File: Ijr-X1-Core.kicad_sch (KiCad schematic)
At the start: 67 parts, among them J1 USB-C_PWR_IN, J2 USB-C_CPU_PROG, J3 USB-C_UART_BRIDGE, Q1 BSC010NE2LS, Q2 BSC010NE2LS, Q3 BSC010NE2LS, Q4 BSC010NE2LS, Q5 BSC010NE2LS, Q6 BSC010NE2LS, Q7 BSC010NE2LS, Q8 BSC010NE2LS, U1 RP2040, U2 W25Q16JVSSIQ, U3 ISL8117FRZ, U4 ISL8117FRZ, U5 ISL8117FRZ, U6 ISL8117FRZ

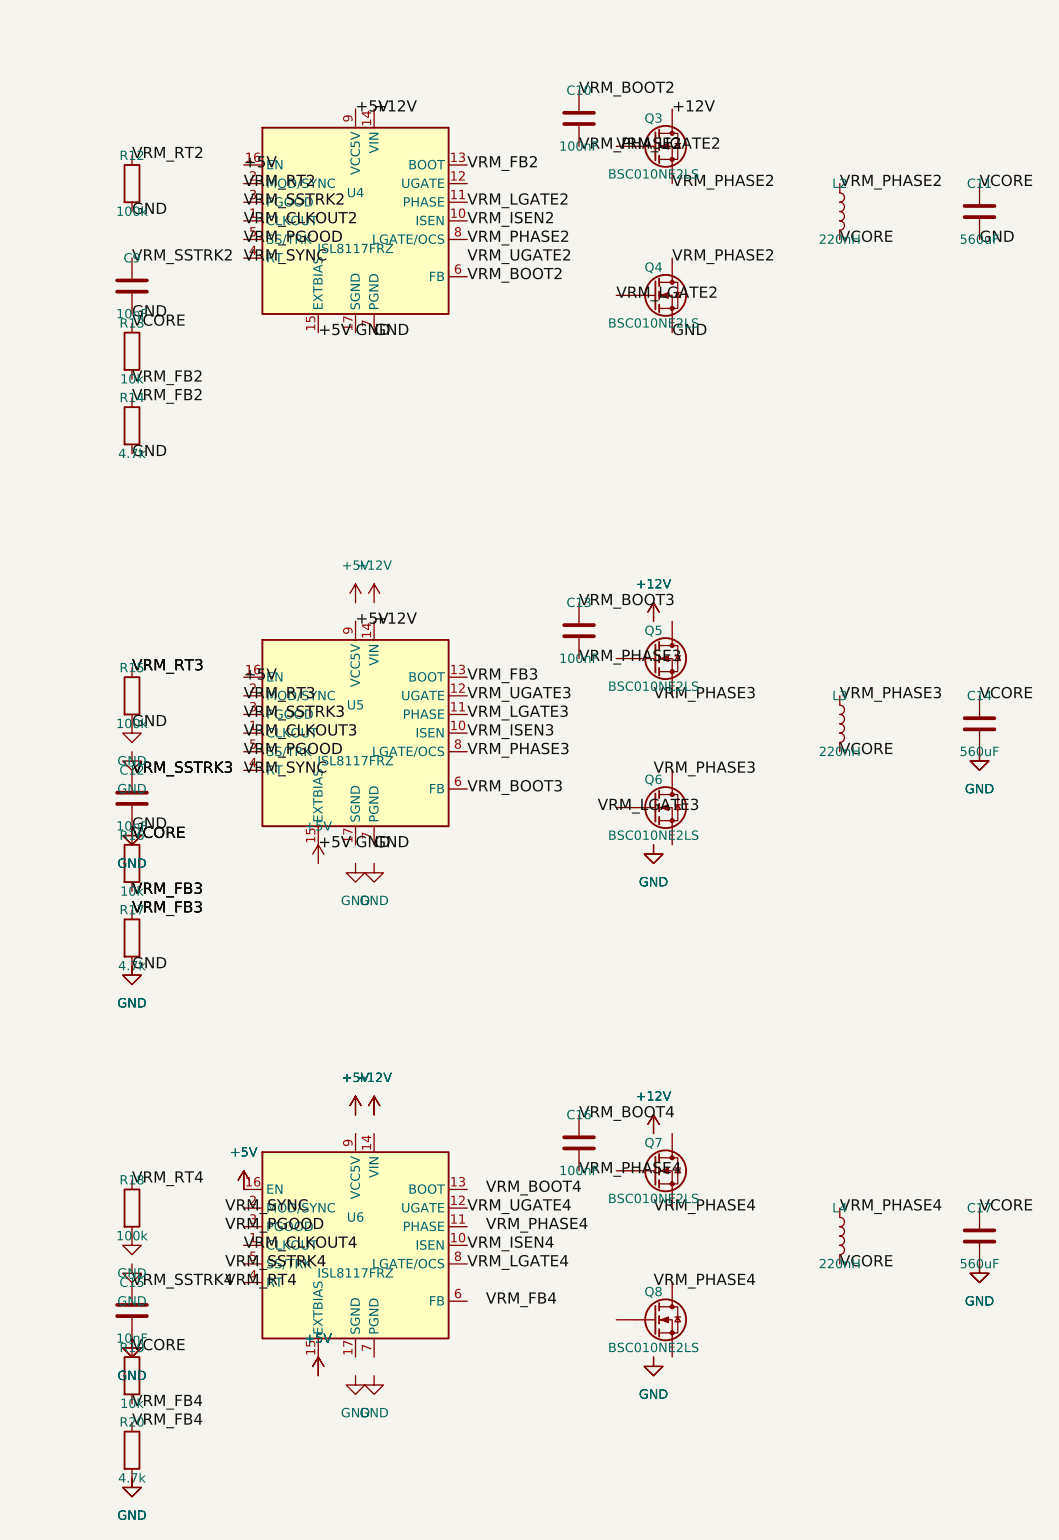
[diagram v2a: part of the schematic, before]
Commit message: Some updates1
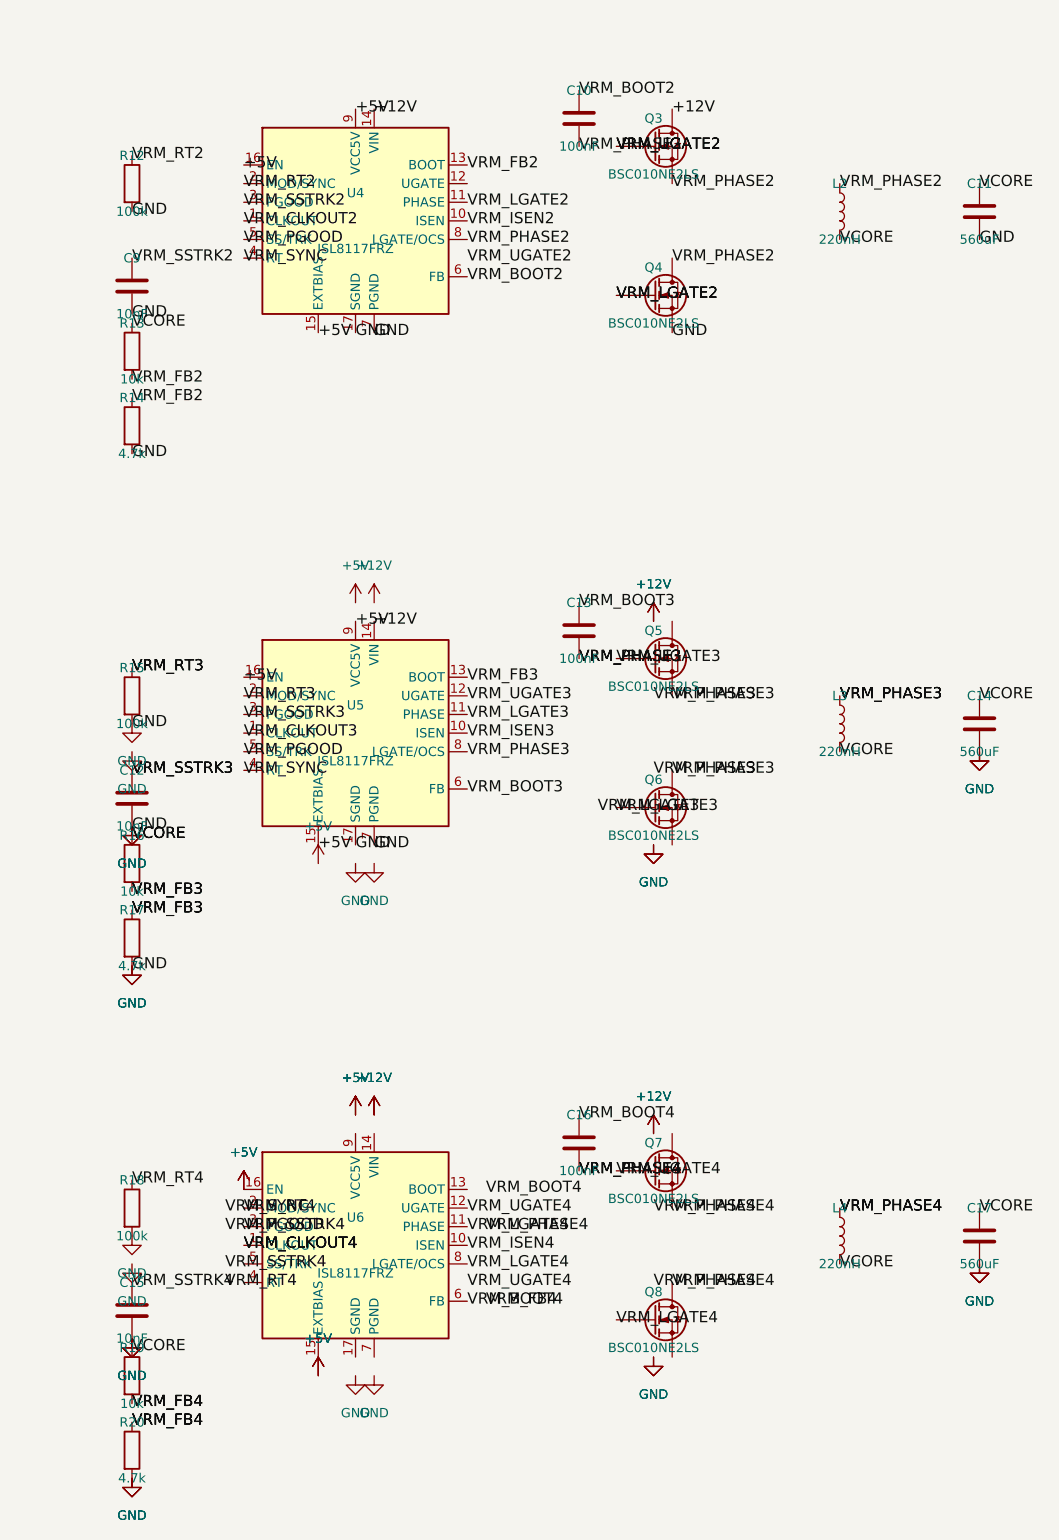
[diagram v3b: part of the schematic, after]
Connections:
- net VRM_BOOT4: now also U6.6 (FB)
- net VRM_LGATE3: now also Q6.G
- net VRM_LGATE4: now also Q8.G, U6.11 (PHASE)
- net VRM_PHASE3: now also Q5.S, Q6.D
- net VRM_PHASE4: now also Q7.S, Q8.D
- net VRM_RT4: now also U6.2 (MOD/SYNC)
- net VRM_SSTRK4: now also U6.3 (PGOOD)
- net VRM_UGATE3: now also Q5.G
- net VRM_UGATE4: now also Q7.G
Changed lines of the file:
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@@
 		)
+	)
+	(label "VRM_RT4"
+		(at 274.32 424.18 0)
+		(effects (font (size 1.524 1.524)))
+	)
+	(label "VRM_SSTRK4"
+		(at 274.32 426.72 0)
+		(effects (font (size 1.524 1.524)))
+	)
+	(label "VRM_CLKOUT4"
+		(at 274.32 429.26 0)
+		(effects (font (size 1.524 1.524)))
+	)
+	(label "VRM_UGATE4"
+		(at 304.8 434.34 0)
+		(effects (font (size 1.524 1.524)))
+	)
+	(label "VRM_LGATE4"
+		(at 304.8 426.72 0)
+		(effects (font (size 1.524 1.524)))
+	)
+	(label "VRM_BOOT4"
+		(at 304.8 436.88 0)
+		(effects (font (size 1.524 1.524)))
+	)
+	(label "VRM_UGATE2"
+		(at 325.12 279.4 0)
+		(effects (font (size 1.524 1.524)))
+	)
+	(label "VRM_LGATE2"
+		(at 325.12 299.72 0)
+		(effects (font (size 1.524 1.524)))
+	)
+	(label "VRM_UGATE3"
+		(at 325.12 349.25 0)
+		(effects (font (size 1.524 1.524)))
+	)
+	(label "VRM_LGATE3"
+		(at 325.12 369.57 0)
+		(effects (font (size 1.524 1.524)))
+	)
+	(label "VRM_UGATE4"
+		(at 325.12 419.1 0)
+		(effects (font (size 1.524 1.524)))
+	)
+	(label "VRM_LGATE4"
+		(at 325.12 439.42 0)
+		(effects (font (size 1.524 1.524)))
+	)
+	(label "VRM_PHASE3"
+		(at 332.74 354.33 0)
+		(effects (font (size 1.524 1.524)))
+	)
+	(label "VRM_PHASE3"
+		(at 332.74 364.49 0)
+		(effects (font (size 1.524 1.524)))
+	)
+	(label "VRM_PHASE3"
+		(at 320.04 349.25 0)
+		(effects (font (size 1.524 1.524)))
+	)
+	(label "VRM_PHASE3"
+		(at 355.6 354.33 0)
+		(effects (font (size 1.524 1.524)))
+	)
+	(label "VRM_PHASE4"
+		(at 332.74 424.18 0)
+		(effects (font (size 1.524 1.524)))
+	)
+	(label "VRM_PHASE4"
+		(at 332.74 434.34 0)
+		(effects (font (size 1.524 1.524)))
+	)
+	(label "VRM_PHASE4"
+		(at 320.04 419.1 0)
+		(effects (font (size 1.524 1.524)))
+	)
+	(label "VRM_PHASE4"
+		(at 355.6 424.18 0)
+		(effects (font (size 1.524 1.524)))
+	)
+	(label "VRM_FB4"
+		(at 259.08 450.85 0)
+		(effects (font (size 1.524 1.524)))
+	)
+	(label "VRM_FB4"
+		(at 259.08 453.39 0)
+		(effects (font (size 1.524 1.524)))
 	)
 	(sheet_instances

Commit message: Some updates1
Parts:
- added J_DIMM1, J_DIMM2: DDR4_SO-DIMM_260, symbol dfdtc_Connector:DDR4_SODIMM_CONN260
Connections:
- net +12V: now also Q5.D, Q7.D, U6.14 (VIN)
- net +5V: now also U6.15 (EXTBIAS), U6.9 (VCC5V)
- net GND: now also Q6.S, Q8.S, U6.17 (SGND), U6.7 (PGND)
- net VRM_BOOT4: now also U6.13 (BOOT); no longer U6.6 (FB)
- net VRM_FB4: now also U6.6 (FB)
- net VRM_LGATE4: no longer U6.11 (PHASE)
- net VRM_PGOOD: now also U6.3 (PGOOD)
- net VRM_PHASE4: now also U6.11 (PHASE)
- net VRM_RT4: now also U6.4 (RT); no longer U6.2 (MOD/SYNC)
- net VRM_SSTRK4: now also U6.5 (SS/TRK); no longer U6.3 (PGOOD)
- net VRM_SYNC: now also U6.2 (MOD/SYNC)
- net VRM_UGATE2: now also U4.12 (UGATE)
